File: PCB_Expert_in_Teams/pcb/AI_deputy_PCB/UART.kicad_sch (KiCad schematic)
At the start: 7 parts, among them IC8 FT231XS-R

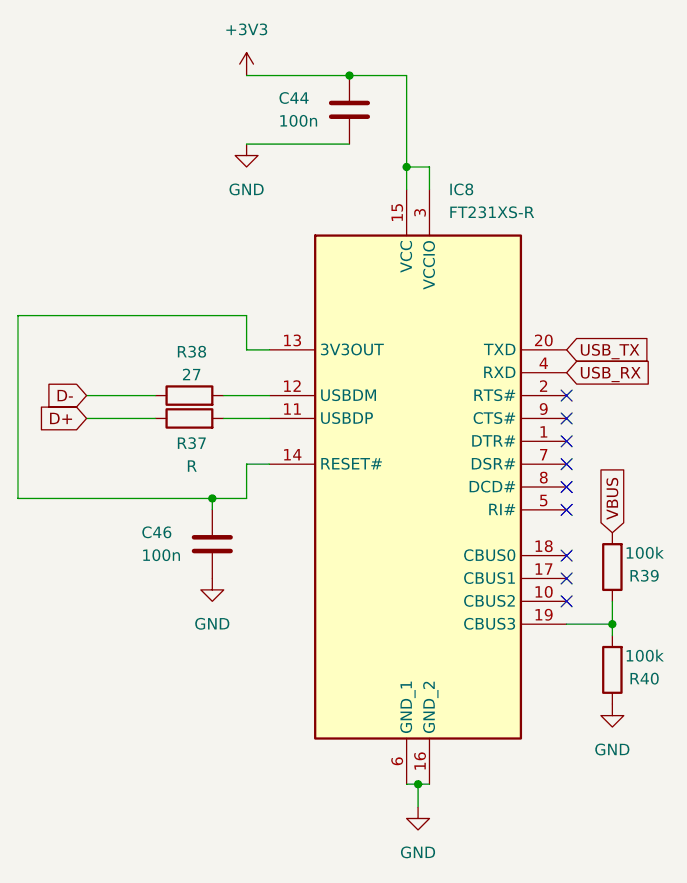
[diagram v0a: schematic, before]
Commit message: fixed small things, push from laptop
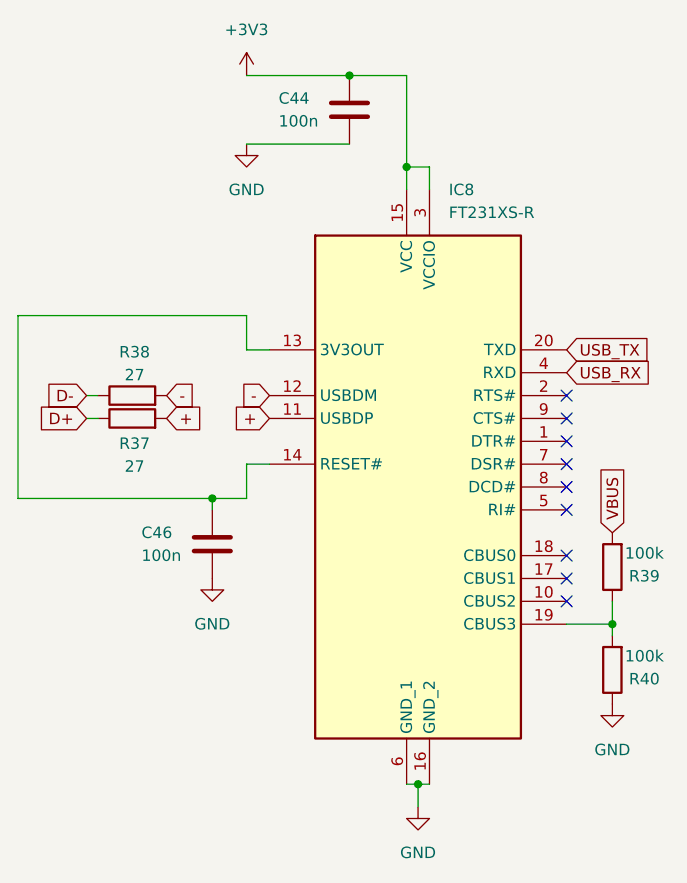
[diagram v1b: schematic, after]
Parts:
- R37: value R -> 27
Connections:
- net +: now reaches IC8.11 (USBDP), R37.2
- net -: now reaches IC8.12 (USBDM), R38.2
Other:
- moved on the sheet: R37, R38
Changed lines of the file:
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@@
-	(wire
-		(pts
-			(xy 127 76.2) (xy 132.08 76.2)
-		)
-		(stroke
-			(width 0)
-			(type default)
-		)
-	)
 	(wire
 		(pts
@@
 	(wire
 		(pts
-			(xy 111.76 76.2) (xy 119.38 76.2)
+			(xy 111.76 76.2) (xy 113.03 76.2)
 		)
 		(stroke
@@
 	(wire
 		(pts
-			(xy 127 78.74) (xy 132.08 78.74)
-		)
-		(stroke
-			(width 0)
-			(type default)
-		)
-	)
-	(wire
-		(pts
 			(xy 129.54 71.12) (xy 129.54 67.31)
 		)
@@
 	(wire
 		(pts
-			(xy 111.76 78.74) (xy 119.38 78.74)
+			(xy 111.76 78.74) (xy 113.03 78.74)
 		)
 		(stroke
@@
 			(width 0)
 			(type default)
+		)
+	)
+	(global_label "-"
+		(shape input)
+		(at 132.08 76.2 180)
+		(fields_autoplaced yes)
+		(effects
+			(font
+				(size 1.27 1.27)
+			)
+			(justify right)
+		)
+		(property "Intersheetrefs" "${INTERSHEET_REFS}"
+			(at 127.5224 76.2 0)
+			(effects
+				(font
+					(size 1.27 1.27)
+				)
+				(justify right)
+				(hide yes)
+			)
+		)
+	)
+	(global_label "+"
+		(shape input)
+		(at 120.65 78.74 0)
+		(fields_autoplaced yes)
+		(effects
+			(font
+				(size 1.27 1.27)
+			)
+			(justify left)
+		)
+		(property "Intersheetrefs" "${INTERSHEET_REFS}"
+			(at 125.2076 78.74 0)
+			(effects
+				(font
+					(size 1.27 1.27)
+				)
+				(justify left)
+				(hide yes)
+			)
+		)
+	)
+	(global_label "-"
+		(shape input)
+		(at 120.65 76.2 0)
+		(fields_autoplaced yes)
+		(effects
+			(font
+				(size 1.27 1.27)
+			)
+			(justify left)
+		)
+		(property "Intersheetrefs" "${INTERSHEET_REFS}"
+			(at 125.2076 76.2 0)
+			(effects
+				(font
+					(size 1.27 1.27)
+				)
+				(justify left)
+				(hide yes)
+			)
 		)
 	)
@@
 				)
 				(justify left)
+				(hide yes)
+			)
+		)
+	)
+	(global_label "+"
+		(shape input)
+		(at 132.08 78.74 180)
+		(fields_autoplaced yes)
+		(effects
+			(font
+				(size 1.27 1.27)
+			)
+			(justify right)
+		)
+		(property "Intersheetrefs" "${INTERSHEET_REFS}"
+			(at 127.5224 78.74 0)
+			(effects
+				(font
+					(size 1.27 1.27)
+				)
+				(justify right)
 				(hide yes)
 			)
@@
 	(symbol
 		(lib_id "Device:R")
-		(at 123.19 78.74 90)
+		(at 116.84 78.74 90)
 		(unit 1)
 		(exclude_from_sim no)
@@
 		(dnp no)
 		(property "Reference" "R37"
-			(at 123.444 81.534 90)
-			(effects
-				(font
-					(size 1.27 1.27)
-				)
-			)
-		)
-		(property "Value" "R"
-			(at 123.444 84.074 90)
+			(at 117.094 81.534 90)
+			(effects
+				(font
+					(size 1.27 1.27)
+				)
+			)
+		)
+		(property "Value" "27"
+			(at 117.094 84.074 90)
 			(effects
 				(font
@@
 		)
 		(property "Footprint" "Resistor_SMD:R_0805_2012Metric_Pad1.20x1.40mm_HandSolder"
-			(at 123.19 80.518 90)
+			(at 116.84 80.518 90)
 			(effects
 				(font
@@
 		)
 		(property "Datasheet" "~"
-			(at 123.19 78.74 0)
+			(at 116.84 78.74 0)
 			(effects
 				(font
@@
 		)
 		(property "Description" "Resistor"
-			(at 123.19 78.74 0)
+			(at 116.84 78.74 0)
 			(effects
 				(font
@@
 	(symbol
 		(lib_id "Device:R")
-		(at 123.19 76.2 90)
+		(at 116.84 76.2 90)
 		(unit 1)
 		(exclude_from_sim no)
@@
 		(dnp no)
 		(property "Reference" "R38"
-			(at 123.444 71.374 90)
+			(at 117.094 71.374 90)
 			(effects
 				(font
@@
 		)
 		(property "Value" "27"
-			(at 123.444 73.914 90)
+			(at 117.094 73.914 90)
 			(effects
 				(font
@@
 		)
 		(property "Footprint" "Resistor_SMD:R_0805_2012Metric_Pad1.20x1.40mm_HandSolder"
-			(at 123.19 77.978 90)
+			(at 116.84 77.978 90)
 			(effects
 				(font
@@
 		)
 		(property "Datasheet" "~"
-			(at 123.19 76.2 0)
+			(at 116.84 76.2 0)
 			(effects
 				(font
@@
 		)
 		(property "Description" "Resistor"
-			(at 123.19 76.2 0)
-			(effects
-				(font
+			(at 116.84 76.2 0)
+			(effects
+				(font
